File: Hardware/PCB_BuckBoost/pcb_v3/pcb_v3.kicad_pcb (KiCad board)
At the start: 2 copper layers, 43 x 69 mm, 44 parts, among them J1 Conn_01x02, J2 Conn_01x02, J3 Conn_01x02, J4 Conn_01x02, U1 MIC3172YM, U2 MIC3172YM

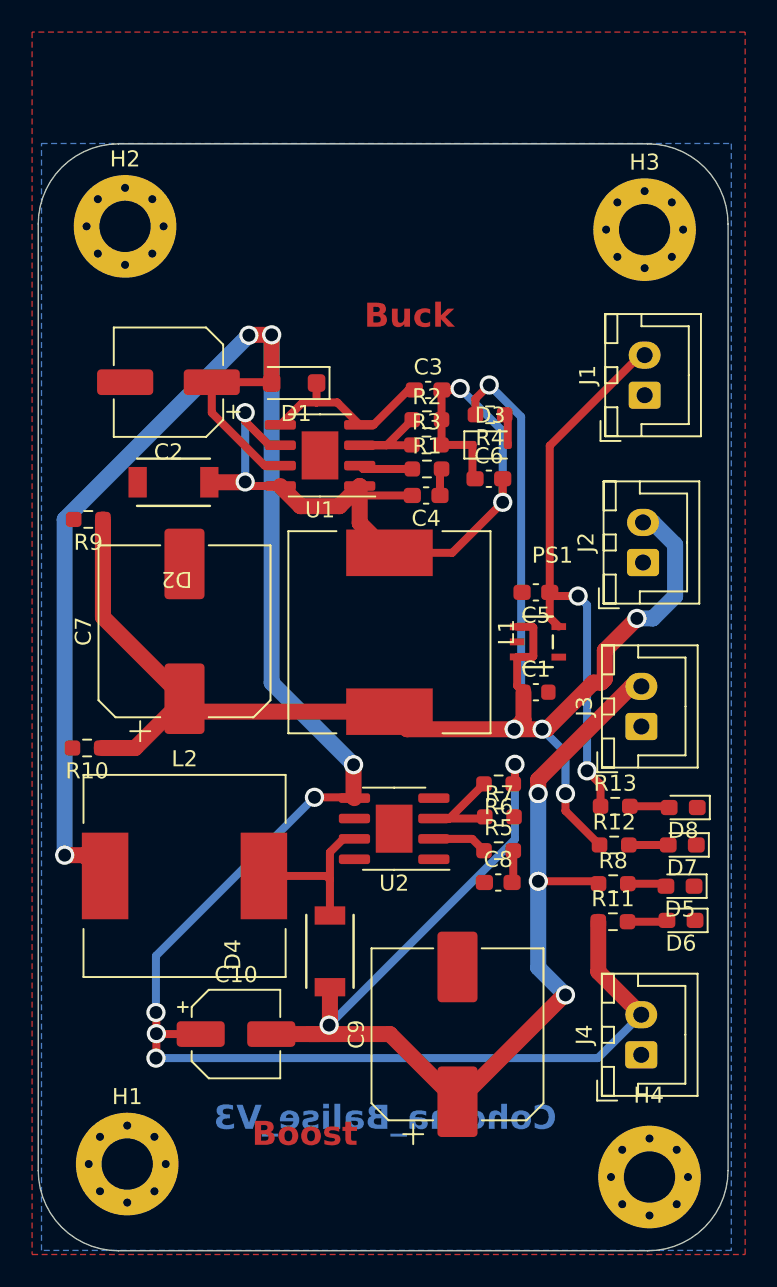
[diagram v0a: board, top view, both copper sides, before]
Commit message: PCB V3 VRAIMENT FINI
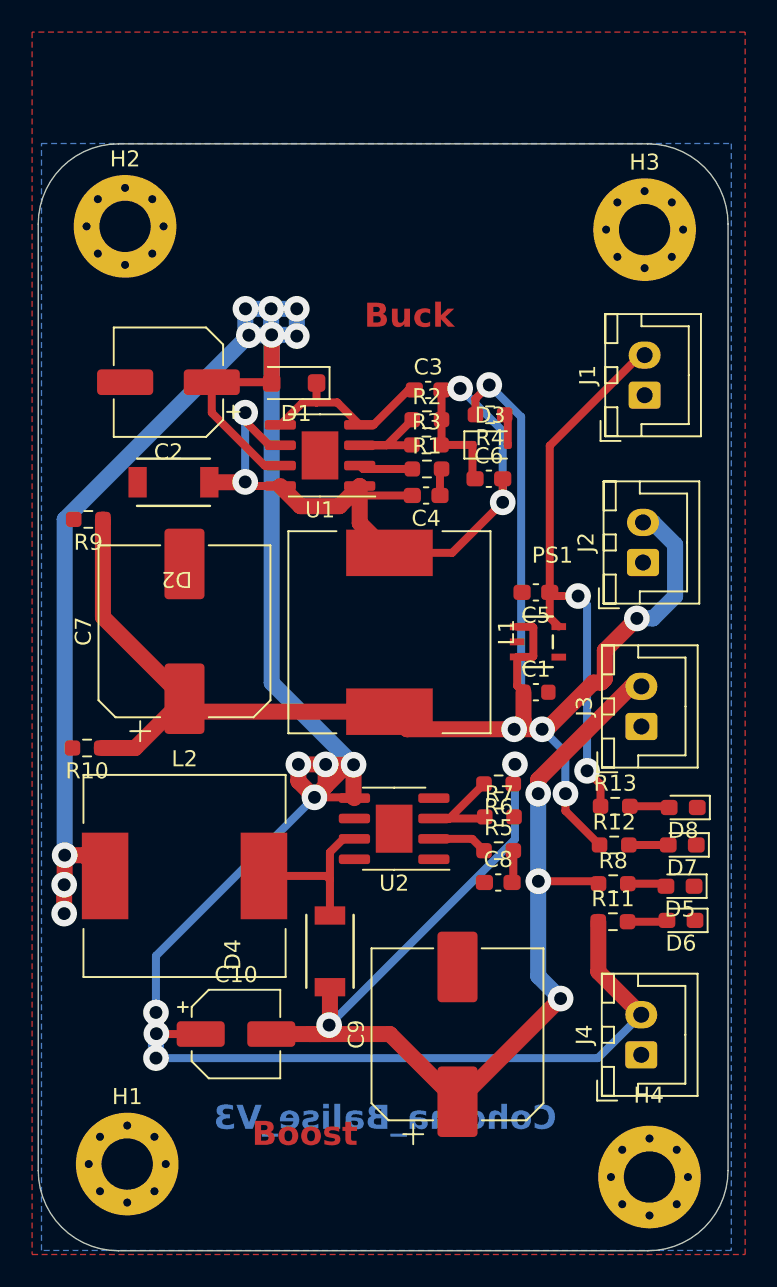
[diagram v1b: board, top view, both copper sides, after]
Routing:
- net +12V: track 150.9 -> 176.0 mm, vias 8 -> 16
- added copper zone on B.Cu, net +12V
- removed copper zone on B.Cu, net GND
